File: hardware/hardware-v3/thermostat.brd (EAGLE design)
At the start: 43.5 x 25.6 mm, 38 parts

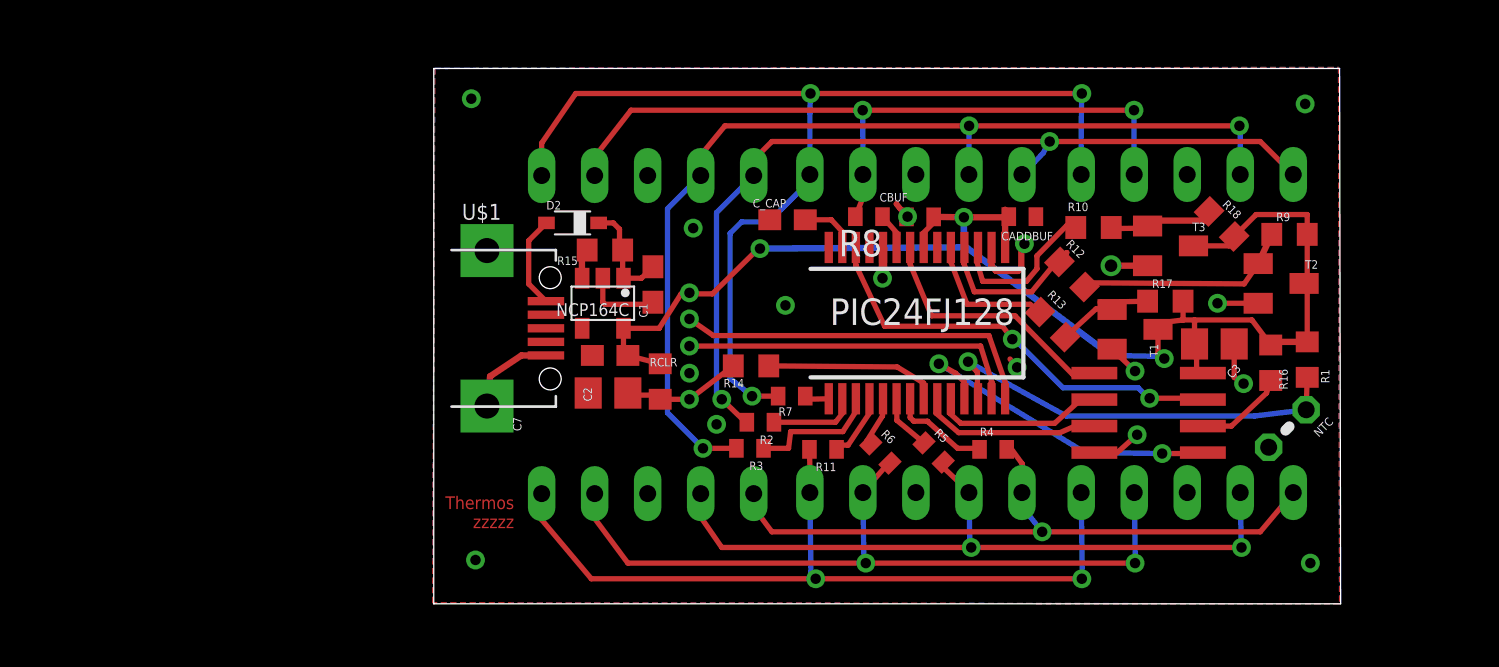
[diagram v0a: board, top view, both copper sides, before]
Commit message: New Layout
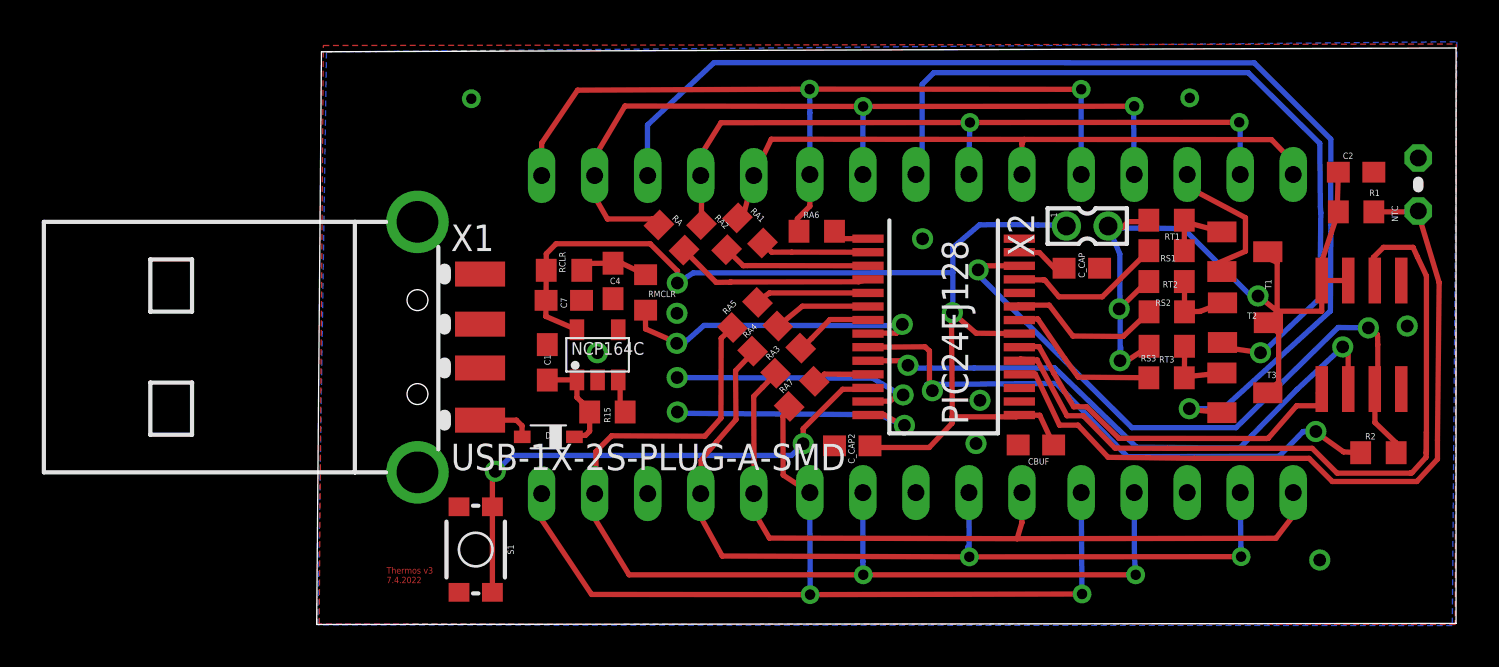
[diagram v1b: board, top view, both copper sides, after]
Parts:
- removed C3: 100n, rcl:C0805
- removed CADDBUF: 100n, eagle-ltspice:C0402
- removed R10, R12, R13, R16: 1k, rcl:R0603
- removed R11, R3, R4, R5, R6, R7, R8: 47, resistor:R0402
- removed R14: 100, rcl:R0603
- removed R17, R18, R9: 10k, rcl:R0603
- removed U$3: MCP4141-103, microchip:SO-08
- added C4, C_CAP2: 100n, eagle-ltspice:C0603
- added RA, RA1, RA2, RA3, RA4, RA5, RA6, RA7: 47, rcl:R0603
- added RMCLR: 100, rcl:R0603
- added RS1, RS2, RS3: 1k, rcl:R0603
- added RT1, RT2, RT3: 10k, rcl:R0603
- added S1: MOMENTARY-SWITCH-SPST-SMD-4.6X2.8MM, SparkFun-Switches:TACTILE_SWITCH_SMD_4.6X2.8MM
- added X1: USB-1X-2S-PLUG-A-SMD, _con-usb:USB-PLUG-A-SMD-2S
- added X2: 332-02, con-garry:332-02
- C2: device rcl:C0805 -> eagle-ltspice:C0603
- CBUF: device eagle-ltspice:C0402 -> eagle-ltspice:C0603
- R2: value 47 -> 1k; device resistor:R0402 -> rcl:R0603
- U$1: value MICRO-USB -> MCP4151; device microusb:MICRO-USB -> microchip:SO-08
- moved U$1 43.6 mm to (36.0, 39.8), turned to 0 degrees
- moved C2 37.4 mm to (35.7, 47.6), turned to 0 degrees
- moved R2 29.6 mm to (36.8, 34.1), turned to 0 degrees
- moved C_CAP 14.3 mm to (22.6, 43.0), turned to 0 degrees
- moved NTC 13.3 mm to (38.7, 47.0), turned to 90 degrees
- moved CBUF 12.3 mm to (20.4, 34.5), turned to 180 degrees
- moved D2 10.3 mm to (-3.01, 34.9)
- moved T3 7.89 mm to (30.4, 37.0)
- moved R15 7.76 mm to (-0.18, 36.1), turned to 180 degrees
- moved R1 7.46 mm to (35.7, 45.7), turned to 180 degrees
- moved RCLR 7.05 mm to (-2.26, 42.9), turned to 180 degrees
- moved T1 6.44 mm to (30.4, 43.8)
- moved C1 6.29 mm to (-3.06, 38.5), turned to 90 degrees
- moved C7 3.45 mm to (-2.27, 41.4), turned to 0 degrees
- moved T2 2.54 mm to (30.4, 40.4)
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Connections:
- removed net N$3: R16.1, U$3.6
- new net 3V3G: C2.1, R1.2, RT1.2, RT2.2, RT3.2, T1.E, T2.E, T3.E, U$1.7, U$1.8, X2.2
- new net N$30: S1.3, S1.4, U$2.12
- net +3V3: now also CBUF.1, C_CAP2.2, X2.1; no longer C3.2, CADDBUF.2, CBUF.2, R1.2, R16.2, R17.2, R18.2, R9.2, T1.E, T2.E, T3.E, U$3.8
- net A: now also RA.1; no longer R8.2
- net B: now also RA6.1; no longer R7.2
- net C: now also RA5.1; no longer R6.2
- net CS: now also U$1.1, U$2.20; no longer U$2.22, U$3.1
- net D: now also RA4.1; no longer R5.2
- net DP: now also RA7.1; no longer R11.2
- net E: now also RA3.1; no longer R4.2
- net F: now also RA2.1; no longer R3.2
- net G: now also RA1.1; no longer R2.2
- net GND: now also C4.2, CBUF.2, C_CAP2.1, S1.1, S1.2, U$1.4, X1.4, X1.S1, X1.S2; no longer C3.1, CADDBUF.1, CBUF.1, U$1.GND1, U$1.GND2, U$3.4
- net IN1: now also NTC.1, R1.1, U$2.18; no longer U$2.11, U$3.5
- net IN2: now also U$1.6, U$2.19; no longer NTC.1, R1.1, U$2.12
- net MCLR: now also C4.1, RMCLR.1; no longer C2.1, R14.1
- net N$12: now also RS3.2, RT3.1; no longer R10.2, R18.1
- net N$14: now also RS2.2, RT2.1; no longer R12.2, R9.1
- net N$16: no longer DIS1.3
- net N$17: no longer DIS2.3
- net N$18: no longer DIS3.3
- net N$5: now also RS1.2, RT1.1; no longer R13.2, R17.1
- net N$6: now also X1.1; no longer U$1.1
- net N$8: now also RMCLR.2; no longer R14.2
- net S1: now also RS1.1, U$2.25; no longer R13.1, U$2.19
- net S2: now also RS2.1, U$2.23; no longer R12.1, U$2.18
- net S3: now also RS3.1, U$2.22; no longer R10.1, U$2.17
- net SCK: now also U$1.2; no longer U$3.2
- net SDI: now also R2.1; no longer U$3.3
- net SDO: now also R2.2, U$1.3; no longer U$3.7
- net _A: now also RA.2, U$2.4; no longer R8.1, U$2.23
- net _B: now also RA6.2; no longer R7.1
- net _C: now also RA5.2; no longer R6.1
- net _D: now also RA4.2; no longer R5.1
- net _DP: now also RA7.2, U$2.11; no longer R11.1, U$2.4
- net _E: now also RA3.2; no longer R4.1
- net _F: now also RA2.2; no longer R3.1
- net _G: now also RA1.2; no longer R2.1
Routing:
- net 3V3G: track 0.00 -> 44.2 mm, vias 0 -> 3
- net N$30: track 0.00 -> 25.8 mm, vias 0 -> 2
- net GND: track 20.6 -> 0.00 mm, vias 13 -> 8
- net IN1: track 17.7 -> 37.9 mm, vias 2 -> 0
- net SDI: track 10.2 -> 29.3 mm, vias 0 -> 2
- net N$16: track 26.5 -> 7.62 mm, vias 1 -> 0
- net SCK: track 9.78 -> 28.6 mm, vias 0 -> 2
- net IN2: track 20.4 -> 39.2 mm, vias 1 -> 0
- net PGD: track 17.8 -> 0.00 mm
- net +3V3: track 71.3 -> 55.0 mm, vias 3 -> 2
- net N$7: track 16.7 -> 1.26 mm, vias 5 -> 0
- net F: track 48.4 -> 35.6 mm, vias 3 -> 2
- net C: track 37.1 -> 49.8 mm
- net N$18: track 44.8 -> 56.3 mm
- net SDO: track 22.3 -> 33.7 mm
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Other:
- board size 43.5 x 25.6 mm -> 54.6 x 27.6 mm
- board text added: "Thermos v3 7.4.2022"
- board text removed: "Thermos zzzzz"
